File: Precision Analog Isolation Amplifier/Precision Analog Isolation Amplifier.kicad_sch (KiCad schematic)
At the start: 58 parts, among them IC1 ADA4899-1YRDZ, J1 Conn_01x03, J2 Conn_01x03, J3 Conn_Coaxial, J4 Conn_Coaxial, Q1 ---, U1 HCNR201, U2 ADA4522, U4 ADA4522

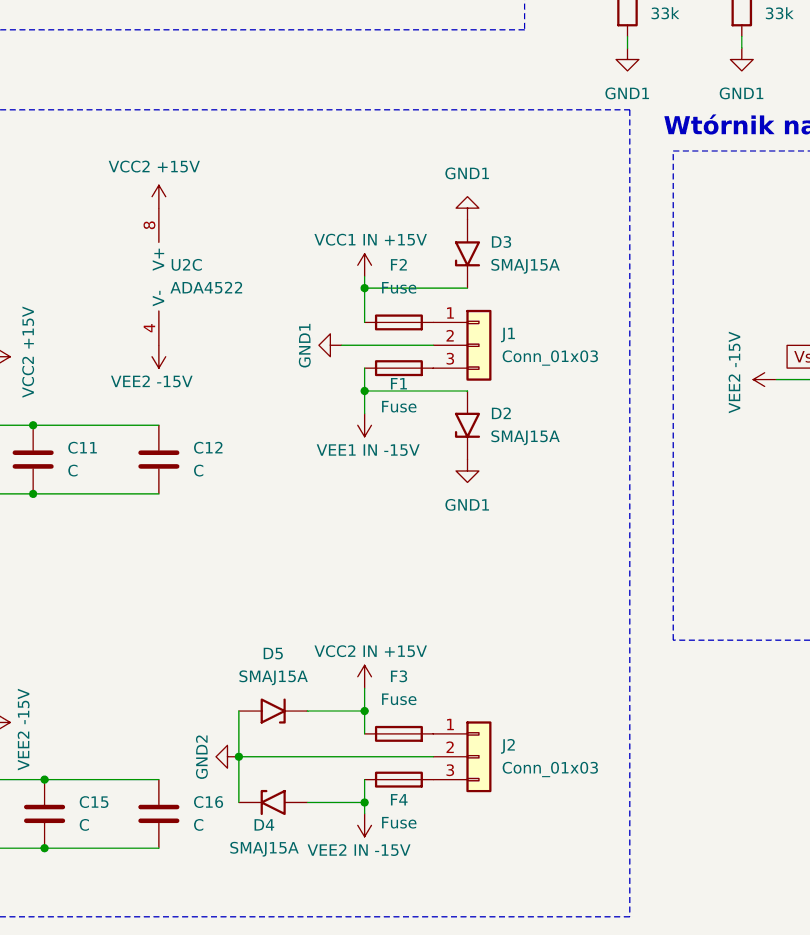
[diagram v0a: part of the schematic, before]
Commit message: Update PCB layout
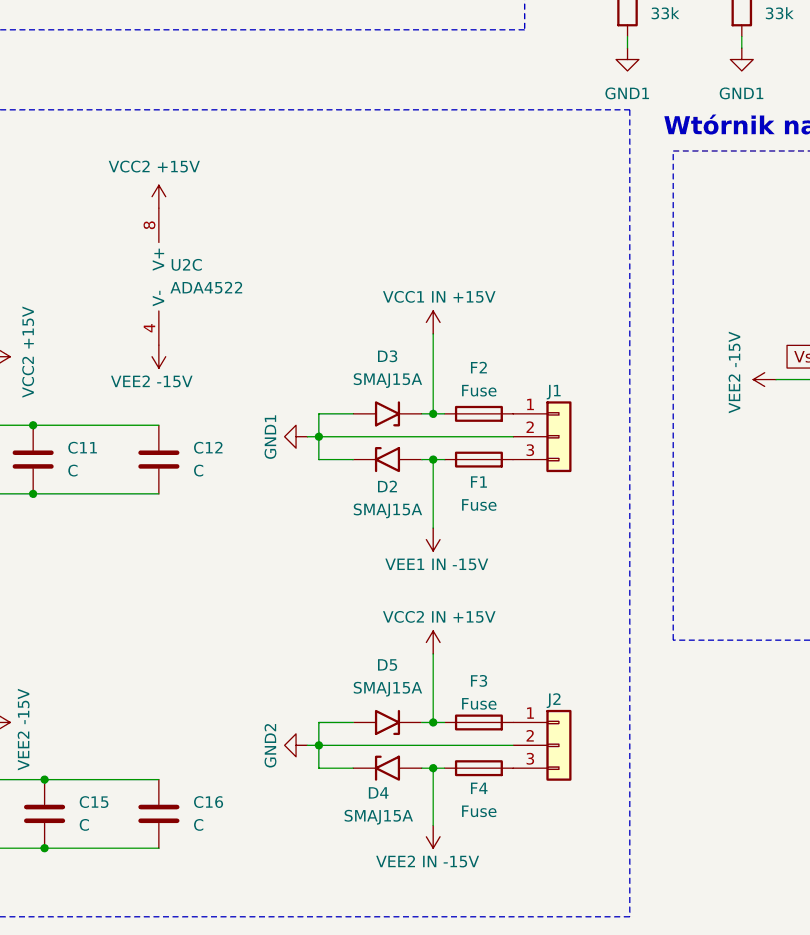
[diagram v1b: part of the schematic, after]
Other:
- moved on the sheet: D2, D3, D4, D5, F1, F2, F3, F4, J1, J2
